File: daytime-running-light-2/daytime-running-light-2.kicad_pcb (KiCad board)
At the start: 2 copper layers, 81.2 x 82.8 mm, 67 parts, among them J1 Conn_01x01_Socket, J2 Conn_01x01_Socket, J3 Conn_01x01_Socket, J4 Conn_01x01_Socket, J5 Conn_01x01_Socket, J6 Conn_01x01_Socket, J7 Conn_01x01_Socket, J8 Conn_01x01_Pin, J9 Conn_01x01_Socket, Q1 BC548, Q2 IRF9540N, Q3 IRFB3004PbF, SW1 SW_SPST, U1 L7812, U2 TLC555xP, U3 L7812, U4 4001, U5 4069, U6 IRS10752LPbF

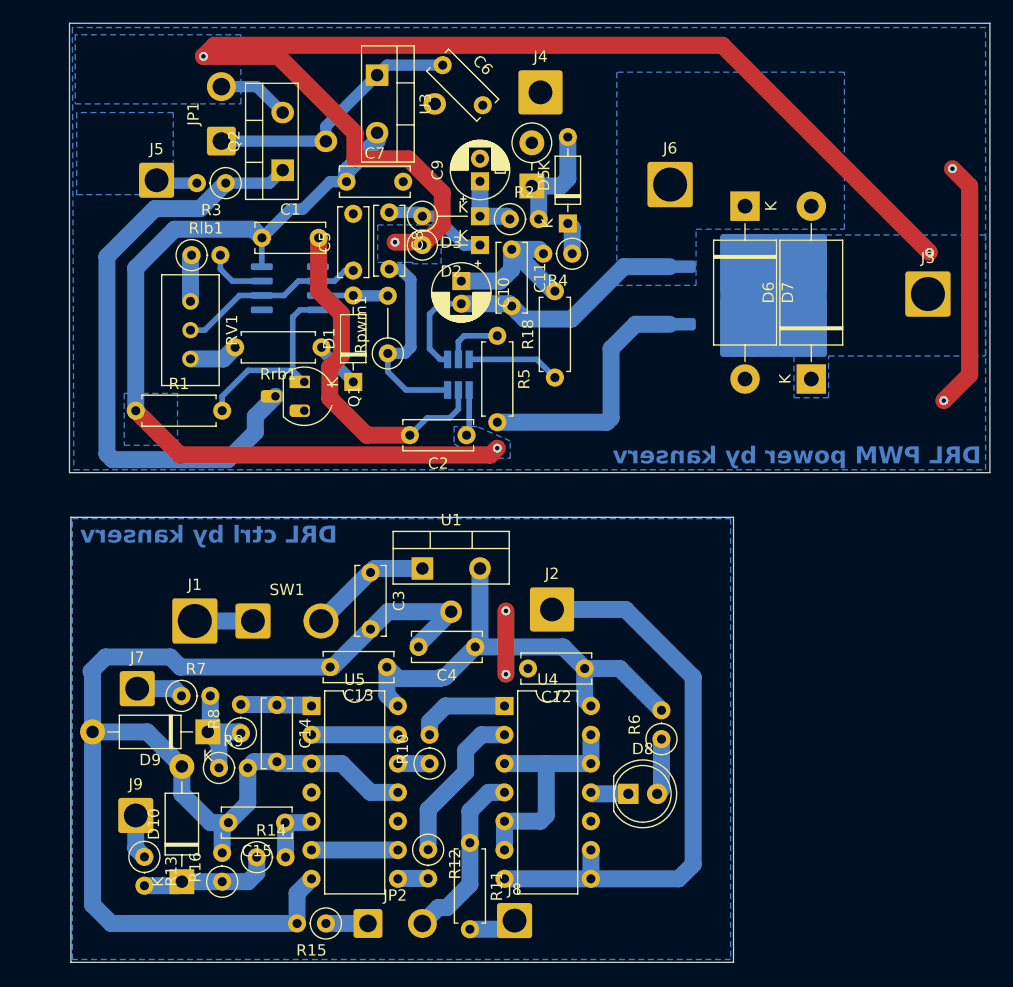
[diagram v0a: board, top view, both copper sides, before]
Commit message: [drl] Fix design rules check
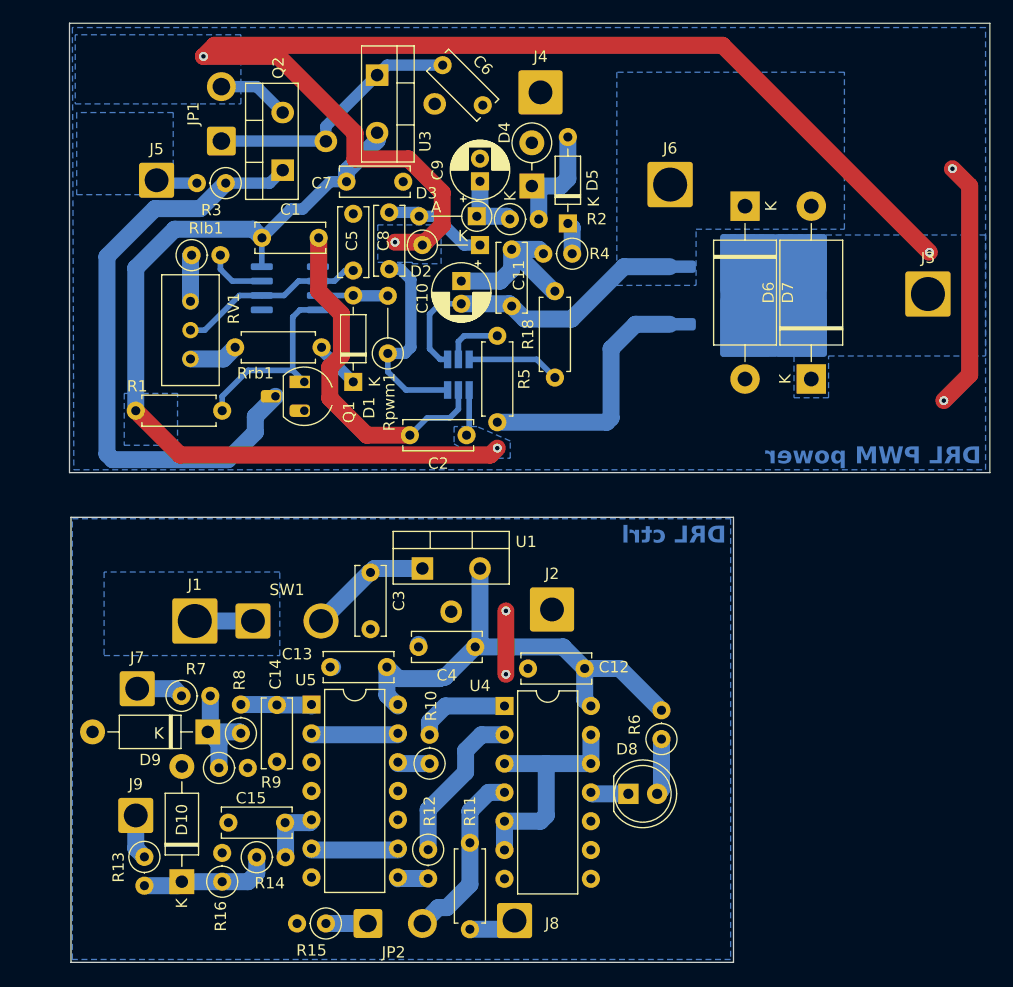
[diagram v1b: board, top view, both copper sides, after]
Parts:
- D3: footprint Diode_THT:D_DO-35_SOD27_P5.08mm_Vertical_KathodeUp -> Diode_THT:D_DO-35_SOD27_P5.08mm_Vertical_AnodeUp
- moved D3 0.28 mm to (59.4, 37.2)
- moved U5 0.13 mm to (44.8, 80.3)
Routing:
- net GND: track 179.2 -> 6.03 mm
- added copper zone on B.Cu, net +BATT
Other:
- board text added: "DRL PWM power"
- board text added: "DRL ctrl"
- board text removed: "DRL PWM power by kanserv"
- board text removed: "DRL ctrl by kanserv"
